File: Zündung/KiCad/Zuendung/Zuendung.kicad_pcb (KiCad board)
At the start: 2 copper layers, 6 parts

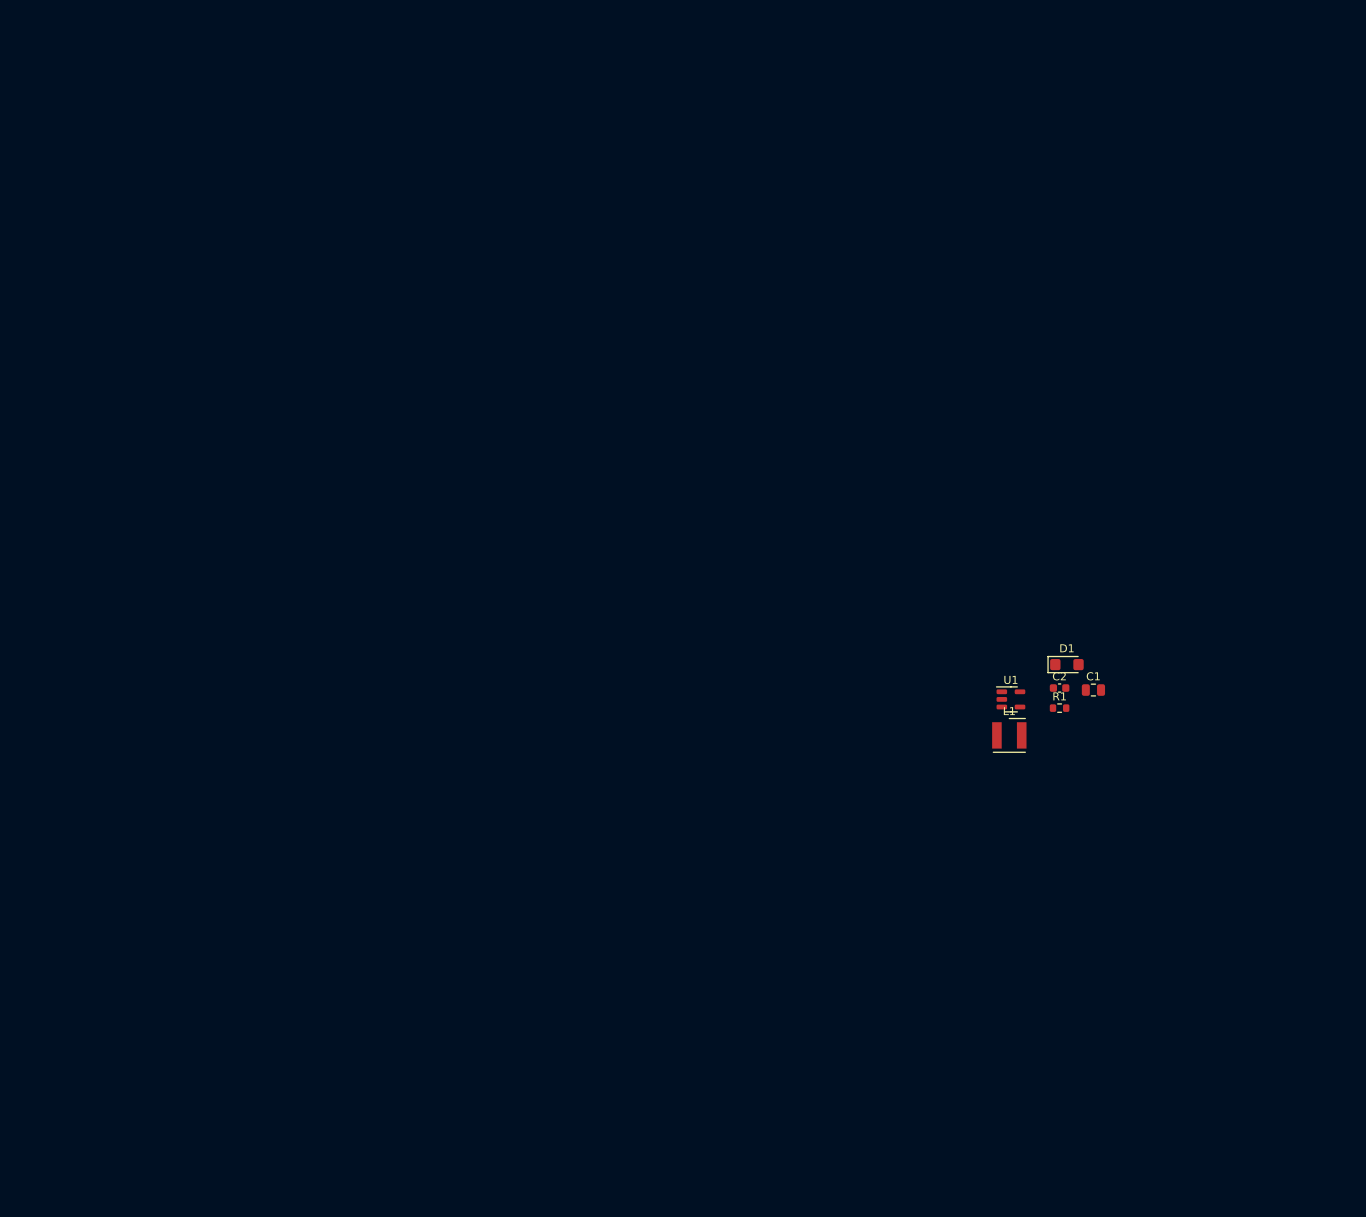
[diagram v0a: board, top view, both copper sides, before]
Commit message: update HW
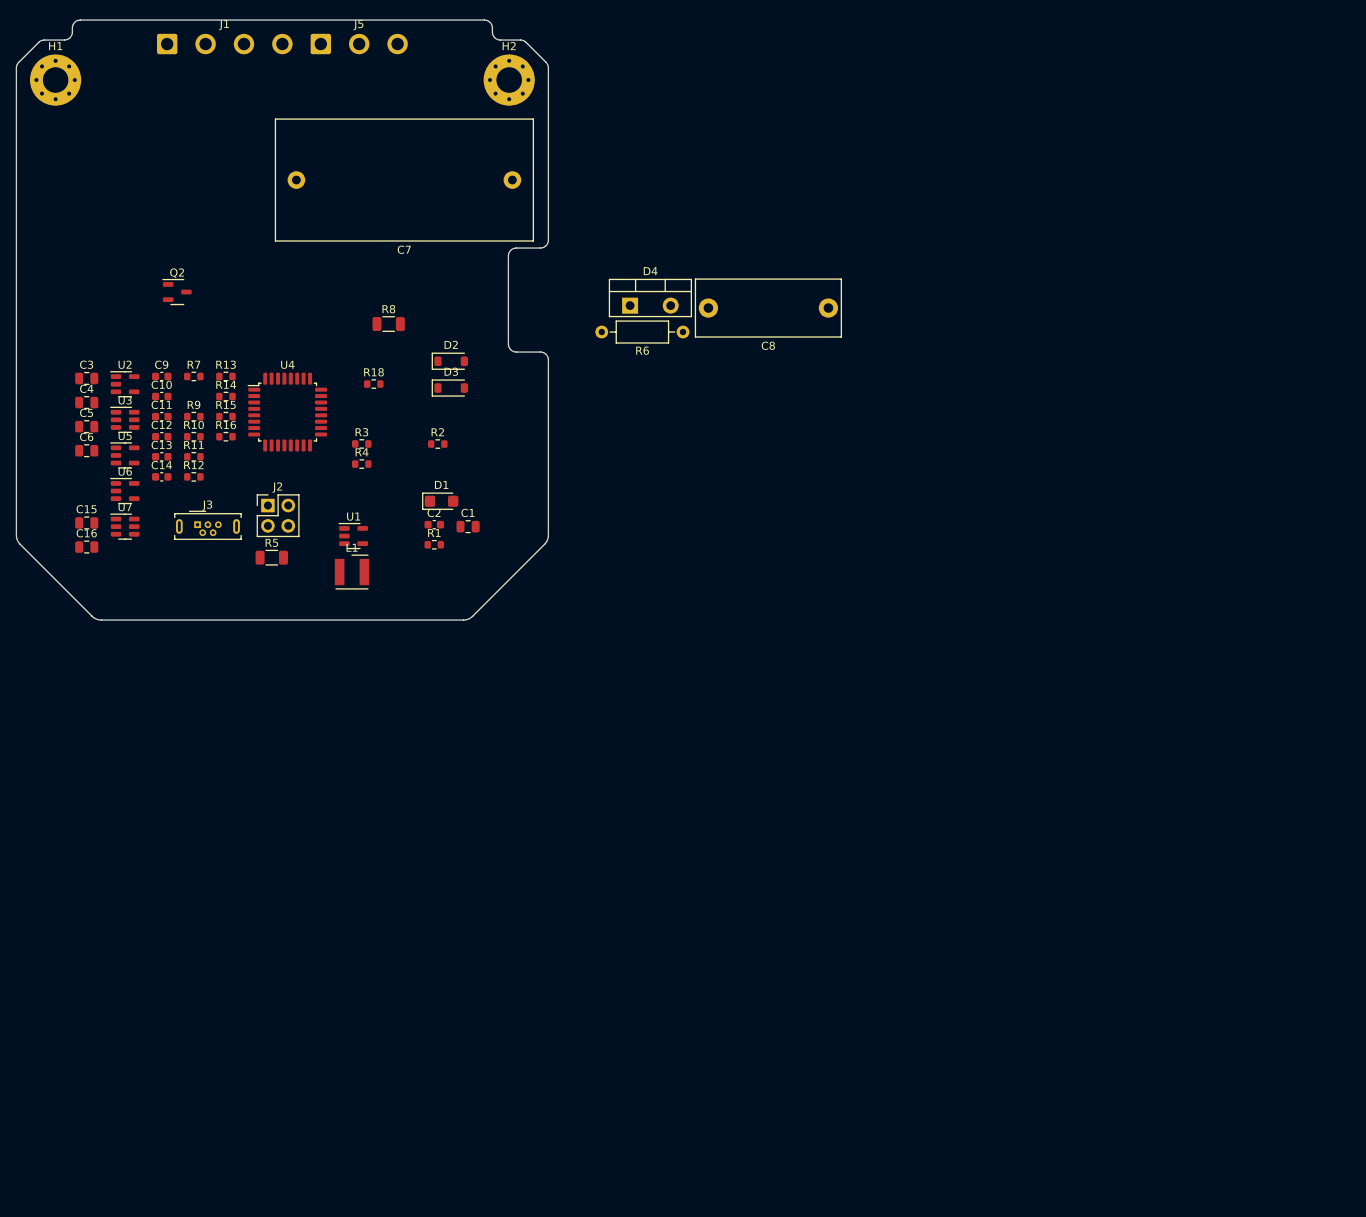
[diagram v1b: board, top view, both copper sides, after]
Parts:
- added C10: 100n, Capacitor_SMD:C_0603_1608Metric, F.Cu at (18.2, 47.1)
- added C11: 100n, Capacitor_SMD:C_0603_1608Metric, F.Cu at (18.2, 49.6)
- added C12: 100n, Capacitor_SMD:C_0603_1608Metric, F.Cu at (18.2, 52.1)
- added C13: 100n, Capacitor_SMD:C_0603_1608Metric, F.Cu at (18.2, 54.6)
- added C14: 100n, Capacitor_SMD:C_0603_1608Metric, F.Cu at (18.2, 57.1)
- added C15: 4.7u, Capacitor_SMD:C_0805_2012Metric, F.Cu at (8.79, 62.9)
- added C16: 4.7u, Capacitor_SMD:C_0805_2012Metric, F.Cu at (8.79, 65.9)
- added C3: 4.7u, Capacitor_SMD:C_0805_2012Metric, F.Cu at (8.79, 44.8)
- added C4: 4.7u, Capacitor_SMD:C_0805_2012Metric, F.Cu at (8.79, 47.8)
- added C5: 100n, Capacitor_SMD:C_0805_2012Metric, F.Cu at (8.79, 50.8)
- added C6: 4.7u, Capacitor_SMD:C_0805_2012Metric, F.Cu at (8.79, 53.8)
- added C7: 150n, Capacitor_THT:C_Rect_L32.0mm_W15.0mm_P27.00mm, F.Cu at (62.0, 20.0)
- added C8: 10n, Capacitor_THT:C_Rect_L18.0mm_W7.0mm_P15.00mm_FKS3_FKP3, F.Cu at (101.5, 36.0)
- added C9: 100n, Capacitor_SMD:C_0603_1608Metric, F.Cu at (18.2, 44.6)
- added D2: DZ6V, Diode_SMD:D_SOD-123, F.Cu at (54.4, 42.6)
- added D3: DZ12V, Diode_SMD:D_SOD-123, F.Cu at (54.4, 46.0)
- added D4: D, Package_TO_SOT_THT:TO-220-2_Vertical, F.Cu at (76.7, 35.7)
- added H1: MountingHole_Pad, MountingHole:MountingHole_3.2mm_M3_Pad_Via, F.Cu at (4.90, 7.50)
- added H2: MountingHole_Pad, MountingHole:MountingHole_3.2mm_M3_Pad_Via, F.Cu at (61.6, 7.50)
- added J1: Conn_01x04, Connector_Wire:SolderWire-0.75sqmm_1x04_P4.8mm_D1.25mm_OD2.3mm, F.Cu at (18.9, 3.00)
- added J2: SWD, Connector_PinHeader_2.54mm:PinHeader_2x02_P2.54mm_Vertical, F.Cu at (31.4, 60.7)
- added J3: USB_B_Micro, Connector_USB:USB_Micro-B_Wuerth_614105150721_Vertical, F.Cu at (22.6, 63.1)
- added J5: Conn_01x03, Connector_Wire:SolderWire-0.75sqmm_1x03_P4.8mm_D1.25mm_OD2.3mm, F.Cu at (38.0, 3.00)
- added Q2: Q_NMOS_DGS, Package_TO_SOT_SMD:SOT-23-3, F.Cu at (20.1, 34.0)
- added R10: 100k, Resistor_SMD:R_0603_1608Metric, F.Cu at (22.2, 52.1)
- added R11: 100k, Resistor_SMD:R_0603_1608Metric, F.Cu at (22.2, 54.6)
- added R12: 1k, Resistor_SMD:R_0603_1608Metric, F.Cu at (22.2, 57.1)
- added R13: 1k, Resistor_SMD:R_0603_1608Metric, F.Cu at (26.2, 44.6)
- added R14: 1k, Resistor_SMD:R_0603_1608Metric, F.Cu at (26.2, 47.1)
- added R15: 1k, Resistor_SMD:R_0603_1608Metric, F.Cu at (26.2, 49.6)
- added R16: 1k, Resistor_SMD:R_0603_1608Metric, F.Cu at (26.2, 52.1)
- added R18: 22, Resistor_SMD:R_0603_1608Metric, F.Cu at (44.7, 45.5)
- added R2: 10k, Resistor_SMD:R_0603_1608Metric, F.Cu at (52.7, 53.0)
- added R3: 40k, Resistor_SMD:R_0603_1608Metric, F.Cu at (43.2, 53.0)
- added R4: 10k, Resistor_SMD:R_0603_1608Metric, F.Cu at (43.2, 55.5)
- added R5: 20m, Resistor_SMD:R_1206_3216Metric, F.Cu at (31.9, 67.2)
- added R6: 10k, Resistor_THT:R_Axial_DIN0207_L6.3mm_D2.5mm_P10.16mm_Horizontal, F.Cu at (83.3, 39.0)
- added R7: 22, Resistor_SMD:R_0603_1608Metric, F.Cu at (22.2, 44.6)
- added R8: 100, Resistor_SMD:R_1206_3216Metric, F.Cu at (46.5, 38.0)
- added R9: 1k, Resistor_SMD:R_0603_1608Metric, F.Cu at (22.2, 49.6)
- added U2: TLV2371DBV, Package_TO_SOT_SMD:SOT-23-5, F.Cu at (13.6, 45.5)
- added U3: USBLC6-2SC6, Package_TO_SOT_SMD:SOT-23-6, F.Cu at (13.6, 50.0)
- added U4: STM32G431K8Tx, Package_QFP:LQFP-32_7x7mm_P0.8mm, F.Cu at (33.9, 49.0)
- added U5: TLV2371DBV, Package_TO_SOT_SMD:SOT-23-5, F.Cu at (13.6, 54.4)
- added U6: TLV2371DBV, Package_TO_SOT_SMD:SOT-23-5, F.Cu at (13.6, 58.9)
- added U7: INA181, Package_TO_SOT_SMD:SOT-23-6, F.Cu at (13.6, 63.3)
- moved L1 84.7 mm to (42.0, 69.0)
- moved U1 84.7 mm to (42.1, 64.5)
- moved C2 80.8 mm to (52.2, 63.1)
- moved R1 80.8 mm to (52.2, 65.6)
- moved C1 80.8 mm to (56.5, 63.3)
- moved D1 80.8 mm to (53.1, 60.1)
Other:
- board outline added: 66.5 x 75 mm

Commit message: update HW
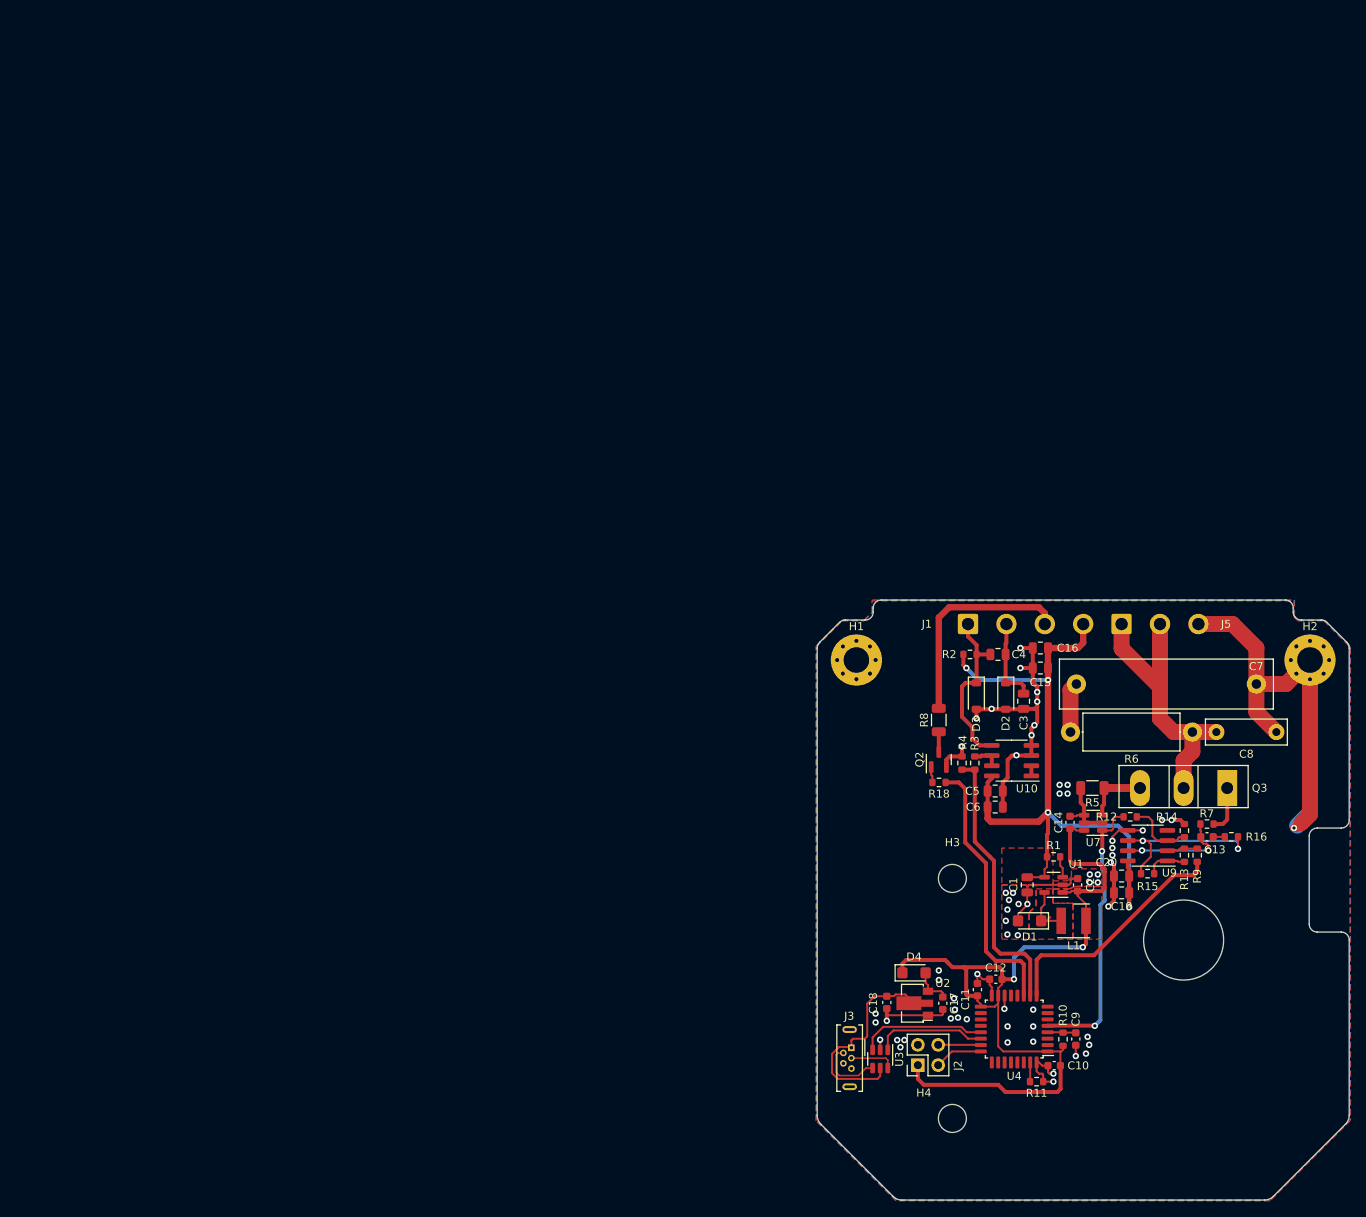
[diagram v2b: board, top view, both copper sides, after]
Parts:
- removed U5, U6: TLV2371DBV, Package_TO_SOT_SMD:SOT-23-5
- added C17: 2.2u, Capacitor_SMD:C_0603_1608Metric, F.Cu at (115.8, 122.9)
- added C18: 1u, Capacitor_SMD:C_0603_1608Metric, F.Cu at (108.8, 122.8)
- added C19: 4.7u, Capacitor_SMD:C_0805_2012Metric, F.Cu at (138.2, 109.1)
- added C20: 100n, Capacitor_SMD:C_0805_2012Metric, F.Cu at (138.2, 107.0)
- added H3: MountingHole, MountingHole:MountingHole_3.5mm, F.Cu at (117.0, 107.3)
- added H4: MountingHole, MountingHole:MountingHole_3.5mm, F.Cu at (117.0, 137.3)
- added Q3: Q_NMOS_GDS, Package_TO_SOT_THT:TO-247-3_Vertical, F.Cu at (151.3, 96.0)
- added U10: TL072, Package_SO:SOIC-8_3.9x4.9mm_P1.27mm, F.Cu at (124.4, 92.6)
- added U9: TL072, Package_SO:SOIC-8_3.9x4.9mm_P1.27mm, F.Cu at (141.4, 103.2)
- C7: footprint Capacitor_THT:C_Rect_L32.0mm_W15.0mm_P27.00mm -> Capacitor_THT:C_Rect_L26.5mm_W6.0mm_P22.50mm_MKS4
- C8: footprint Capacitor_THT:C_Rect_L18.0mm_W7.0mm_P15.00mm_FKS3_FKP3 -> Capacitor_THT:C_Rect_L10.0mm_W3.0mm_P7.50mm_MKS4
- D4: value D -> 1A/60V; footprint Package_TO_SOT_THT:TO-220-2_Vertical -> Diode_SMD:D_SMF
- Q2: value Q_NMOS_DGS -> DMN6140L; footprint Package_TO_SOT_SMD:SOT-23-3 -> Package_TO_SOT_SMD:SOT-23
- R6: value 10k -> 3.9; footprint Resistor_THT:R_Axial_DIN0207_L6.3mm_D2.5mm_P10.16mm_Horizontal -> Resistor_THT:R_Axial_DIN0414_L11.9mm_D4.5mm_P15.24mm_Horizontal
- R8: value 100 -> 680
- U2: value TLV2371DBV -> AP2204RA-3.3; footprint Package_TO_SOT_SMD:SOT-23-5 -> Package_TO_SOT_SMD:SOT-89-3
- moved C9 141.1 mm to (132.4, 127.4), turned to 90 degrees
- moved C10 139.4 mm to (129.7, 130.7)
- moved C13 139.0 mm to (148.8, 102.1)
- moved R7 138.4 mm to (148.8, 100.5)
- moved R9 136.9 mm to (147.6, 104.4), turned to -90 degrees
- moved R16 135.3 mm to (151.9, 102.1)
- moved R13 133.9 mm to (146.0, 104.4), turned to 90 degrees
- moved R10 132.2 mm to (130.8, 127.4), turned to 90 degrees
- moved R14 131.5 mm to (146.0, 101.3), turned to 90 degrees
- moved R11 131.1 mm to (127.5, 132.7), turned to 180 degrees
- moved R15 128.6 mm to (141.4, 106.7)
- moved U7 126.5 mm to (134.6, 100.3), turned to 180 degrees
- moved U2 125.2 mm to (112.0, 122.9), turned to 180 degrees
- moved C11 124.6 mm to (120.1, 121.2), turned to -90 degrees
- moved R12 124.5 mm to (139.2, 99.6)
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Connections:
- C2 pad 1: +3.3V -> +3V3
- C7 pad 2: Net-(D4-K) -> Net-(C7-Pad2)
- D4 pad 1: Net-(D4-K) -> +3V3
- D4 pad 2: Ignition -> Net-(D4-A)
- L1 pad 2: +3.3V -> +3V3
- Q2 pad 1: Net-(Q2-D) -> Net-(Q2-G)
- Q2 pad 2: Net-(Q2-G) -> GND
- Q2 pad 3: GND -> Net-(Q2-D)
- R3 pad 1: Net-(U2--) -> Net-(U10B--)
- R6 pad 2: Net-(D4-K) -> Net-(C7-Pad2)
- U1 pad 1: +3.3V -> +3V3
- U2 pad 1: Net-(U2--) -> GND
- U2 pad 2: GND -> VBUS
- U2 pad 3: SpeedSignalPlus -> Net-(D4-A)
- U4 pad 10: unconnected-(U4-PA5-Pad10) -> Tacho
- U4 pad 6: Tacho -> unconnected-(U4-PA1-Pad6)
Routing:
- net GND: track 0.00 -> 171.6 mm, vias 0 -> 63
- net +3V3: track 0.00 -> 106.4 mm, vias 0 -> 2
- net VCC: track 0.00 -> 90.6 mm, vias 0 -> 4
- net Ignition: track 0.00 -> 46.4 mm
- net ISens: track 0.00 -> 35.1 mm, vias 0 -> 2
- net Tacho: track 0.00 -> 34.5 mm
- net RelayOutput: track 0.00 -> 33.5 mm
- net USet: track 0.00 -> 30.4 mm
- net VBUS: track 0.00 -> 28.4 mm
- net FuelRelay: track 0.00 -> 26.8 mm
- net Net-(U9B--): track 0.00 -> 21.5 mm, vias 0 -> 2
- net SpeedSignalPlus: track 0.00 -> 21.3 mm
- net /USB_DM: track 0.00 -> 15.9 mm
- net /USB_DP: track 0.00 -> 14.1 mm
- net Net-(C13-Pad1): track 0.00 -> 14.0 mm, vias 0 -> 2
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- added copper zone on F.Cu, net +3V3
- added copper zone on B.Cu, net GND
- added copper zone on F.Cu, net GND
- added copper zone on F.Cu, net Net-(D1-K)
- added copper zone on F.Cu, net VCC
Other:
- outline, holes or cut-outs redrawn
